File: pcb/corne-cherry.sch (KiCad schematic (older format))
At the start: 145 parts, among them J1 MJ-4PP-9, J2 OLED, J3 MJ-4PP-9, J4 OLED, J5 Conn_01x01_Male, J6 Conn_01x01_Male, P1 Conn_01x03, P3 Conn_01x03, SW1 SW_PUSH, SW10 SW_PUSH, SW11 SW_PUSH, SW12 SW_PUSH, SW13 SW_PUSH, SW14 SW_PUSH, SW15 SW_PUSH, SW16 SW_PUSH, SW17 SW_PUSH, SW18 SW_PUSH, SW19 SW_PUSH, SW2 SW_PUSH, SW20 SW_PUSH, SW21 SW_PUSH, SW22 SW_PUSH, SW23 SW_PUSH, SW24 SW_PUSH, SW25 SW_PUSH, SW26 SW_PUSH, SW27 SW_PUSH, SW28 SW_PUSH, SW29 SW_PUSH, SW3 SW_PUSH, SW30 SW_PUSH, SW31 SW_PUSH, SW32 SW_PUSH, SW33 SW_PUSH, SW34 SW_PUSH, SW35 SW_PUSH, SW36 SW_PUSH, SW37 SW_PUSH, SW38 SW_PUSH, SW39 SW_PUSH, SW4 SW_PUSH, SW40 SW_PUSH, SW41 SW_PUSH, SW42 SW_PUSH, SW43 Rotary_Encoder_Switch, SW5 SW_PUSH, SW6 SW_PUSH, SW7 SW_PUSH, SW8 SW_PUSH, SW9 SW_PUSH, U1 ProMicro, U2 ProMicro

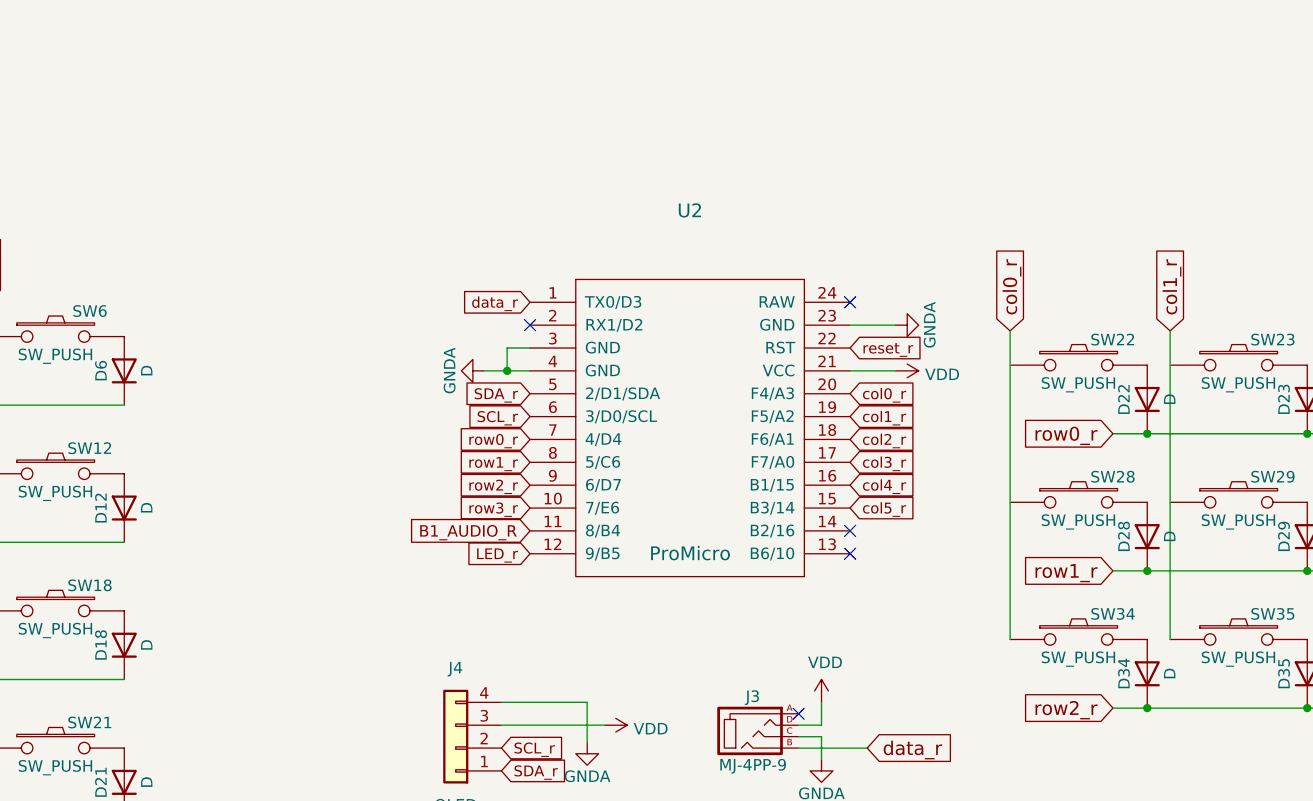
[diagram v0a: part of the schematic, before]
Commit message: Finish PCB
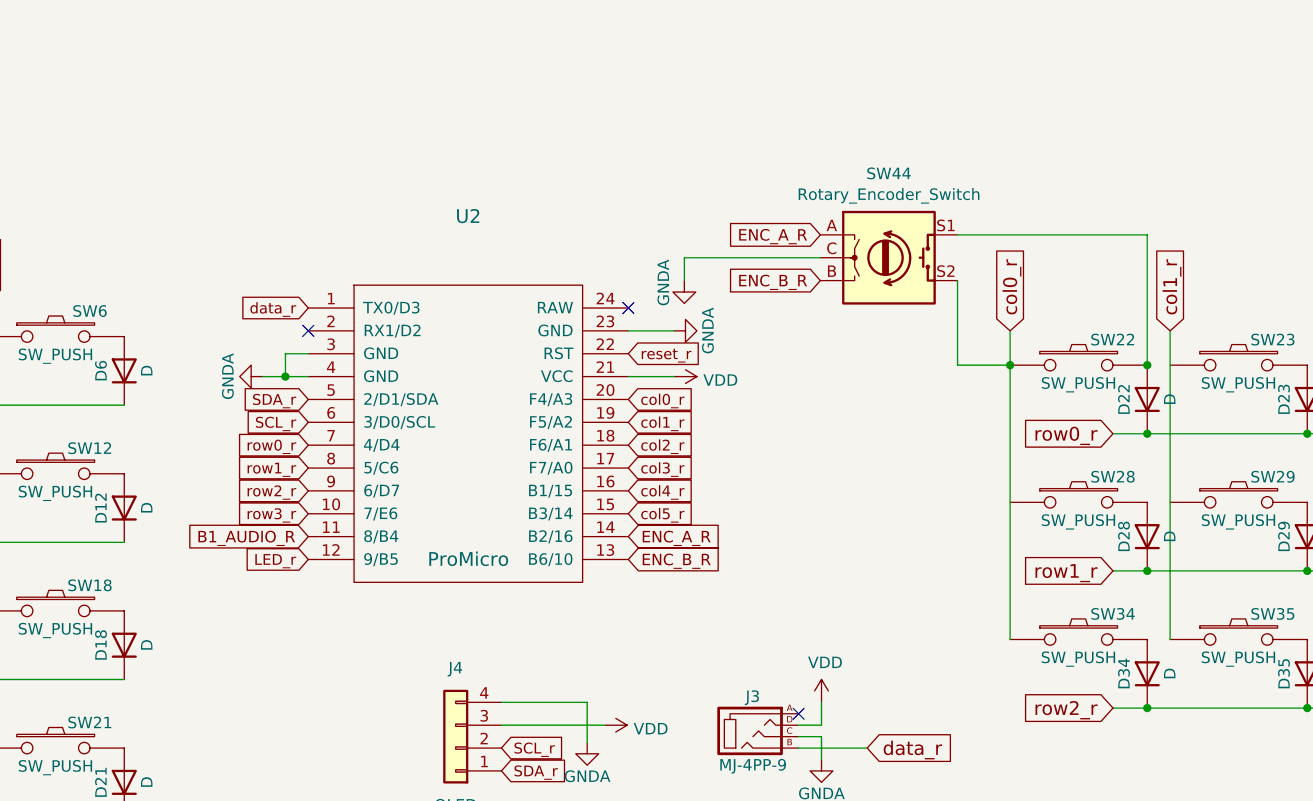
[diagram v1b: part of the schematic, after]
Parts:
- added SW44: Rotary_Encoder_Switch, Keebio-Parts:RotaryEncoder_EC11-no-legs, symbol Device:Rotary_Encoder_Switch
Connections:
- net GNDA: now also SW44.C
- net col0_r: now also SW22.1, SW44.S2
- net ENC_B_R: now reaches U2.13 (B6/10)
- net ENC_B_R: now also SW44.B
- net ENC_A_R: now reaches U2.14 (B2/16)
- net ENC_A_R: now also SW44.A
- net at D22.2 (A), SW22.2: now also SW44.S1
- no-connect marks 13 -> 11
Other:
- moved on the sheet: U2
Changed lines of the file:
@@
 L power:GNDA #PWR017
 U 1 1 5C25F963
-P 11075 1225
-F 0 "#PWR017" H 11075 975 50  0001 C CNN
-F 1 "GNDA" H 11075 1075 50  0000 C CNN
-F 2 "" H 11075 1225 50  0001 C CNN
-F 3 "" H 11075 1225 50  0001 C CNN
-	1    11075 1225
+P 10105 1250
+F 0 "#PWR017" H 10105 1000 50  0001 C CNN
+F 1 "GNDA" H 10105 1100 50  0000 C CNN
+F 2 "" H 10105 1250 50  0001 C CNN
+F 3 "" H 10105 1250 50  0001 C CNN
+	1    10105 1250
 	0    -1   -1   0
 $EndComp
@@
 L power:GNDA #PWR018
 U 1 1 5C25F969
-P 9275 1425
-F 0 "#PWR018" H 9275 1175 50  0001 C CNN
-F 1 "GNDA" H 9275 1275 50  0000 C CNN
-F 2 "" H 9275 1425 50  0001 C CNN
-F 3 "" H 9275 1425 50  0001 C CNN
-	1    9275 1425
+P 8305 1450
+F 0 "#PWR018" H 8305 1200 50  0001 C CNN
+F 1 "GNDA" H 8305 1300 50  0000 C CNN
+F 2 "" H 8305 1450 50  0001 C CNN
+F 3 "" H 8305 1450 50  0001 C CNN
+	1    8305 1450
 	0    1    1    0
 $EndComp
-Text GLabel 10875 1625 2    47   Input ~ 0
+Text GLabel 9905 1650 2    47   Input ~ 0
 col1_r
-Text GLabel 10875 1725 2    47   Input ~ 0
+Text GLabel 9905 1750 2    47   Input ~ 0
 col2_r
-Text GLabel 10875 1825 2    47   Input ~ 0
+Text GLabel 9905 1850 2    47   Input ~ 0
 col3_r
-Text GLabel 10875 1925 2    47   Input ~ 0
+Text GLabel 9905 1950 2    47   Input ~ 0
 col4_r
-Text GLabel 10875 2025 2    47   Input ~ 0
+Text GLabel 9905 2050 2    47   Input ~ 0
 col5_r
-Text GLabel 9475 2025 0    47   Input ~ 0
+Text GLabel 8505 2050 0    47   Input ~ 0
 row3_r
-Text GLabel 9475 1925 0    47   Input ~ 0
+Text GLabel 8505 1950 0    47   Input ~ 0
 row2_r
-Text GLabel 9475 1825 0    47   Input ~ 0
+Text GLabel 8505 1850 0    47   Input ~ 0
 row1_r
-Text GLabel 9475 1725 0    47   Input ~ 0
+Text GLabel 8505 1750 0    47   Input ~ 0
 row0_r
 $Comp
@@
 	1    0    0    -1
 $EndComp
-Text GLabel 9475 2225 0    47   Input ~ 0
+Text GLabel 8505 2250 0    47   Input ~ 0
 LED_r
-Text GLabel 9475 1125 0    47   Input ~ 0
+Text GLabel 8505 1150 0    47   Input ~ 0
 data_r
 $Comp
@@
 Text GLabel 10950 3075 2    60   Input ~ 0
 data_r
-Text GLabel 10875 1325 2    47   Input ~ 0
+Text GLabel 9905 1350 2    47   Input ~ 0
 reset_r
 Text GLabel 9375 3900 0    60   Input ~ 0
 reset_r
-NoConn ~ 9475 1225
-Text GLabel 10875 1525 2    47   Input ~ 0
+NoConn ~ 8505 1250
+Text GLabel 9905 1550 2    47   Input ~ 0
 col0_r
-NoConn ~ 10875 2125
-Text GLabel 9475 1525 0    47   Input ~ 0
+Text GLabel 8505 1550 0    47   Input ~ 0
 SDA_r
-Text GLabel 9475 1625 0    47   Input ~ 0
+Text GLabel 8505 1650 0    47   Input ~ 0
 SCL_r
 $Comp
@@
 Text GLabel 9350 3175 2    47   Input ~ 0
 SDA_r
-NoConn ~ 10875 1125
+NoConn ~ 9905 1150
 $Comp
 L kbd:MJ-4PP-9 J3
@@
 	12025 1700 12175 1700
 Wire Wire Line
-	9375 1325 9375 1425
-Connection ~ 9375 1425
-Wire Wire Line
-	9475 1325 9375 1325
-Wire Wire Line
-	9275 1425 9375 1425
+	8405 1350 8405 1450
+Connection ~ 8405 1450
+Wire Wire Line
+	8505 1350 8405 1350
+Wire Wire Line
+	8305 1450 8405 1450
 Connection ~ 12175 2900
 Connection ~ 12875 2900
@@
 Connection ~ 14975 1700
 Wire Wire Line
-	10875 1225 11075 1225
-Wire Wire Line
-	10875 1425 11075 1425
+	9905 1250 10105 1250
+Wire Wire Line
+	9905 1450 10105 1450
 Wire Wire Line
 	10650 3075 10950 3075
@@
 	14975 3500 15675 3500
 Wire Wire Line
-	9375 1425 9475 1425
+	8405 1450 8505 1450
 Wire Wire Line
 	12175 2900 12875 2900
@@
 L power:VDD #PWR019
 U 1 1 5C714C7F
-P 11075 1425
-F 0 "#PWR019" H 11075 1275 50  0001 C CNN
-F 1 "VDD" V 11092 1553 50  0000 L CNN
-F 2 "" H 11075 1425 50  0001 C CNN
-F 3 "" H 11075 1425 50  0001 C CNN
-	1    11075 1425
+P 10105 1450
+F 0 "#PWR019" H 10105 1300 50  0001 C CNN
+F 1 "VDD" V 10122 1578 50  0000 L CNN
+F 2 "" H 10105 1450 50  0001 C CNN
+F 3 "" H 10105 1450 50  0001 C CNN
+	1    10105 1450
 	0    1    1    0
 $EndComp
@@
 	5000 1125 5000 2475
 Wire Wire Line
-	11575 1250 11575 2600
+	11575 1250 11575 1400
 Wire Wire Line
 	12275 1250 12275 2600
@@
 L kbd:ProMicro U2
 U 1 1 5C25F857
-P 10175 1675
-F 0 "U2" H 10175 2625 60  0000 C CNN
-F 1 "ProMicro" H 10175 1125 60  0000 C CNN
-F 2 "kbd:ProMicro_v3" H 10275 625 60  0001 C CNN
-F 3 "" H 10275 625 60  0000 C CNN
-	1    10175 1675
-	1    0    0    -1
-$EndComp
-NoConn ~ 10875 2225
+P 9205 1700
+F 0 "U2" H 9205 2650 60  0000 C CNN
+F 1 "ProMicro" H 9205 1150 60  0000 C CNN
+F 2 "kbd:ProMicro_v3" H 9305 650 60  0001 C CNN
+F 3 "" H 9305 650 60  0000 C CNN
+	1    9205 1700
+	1    0    0    -1
+$EndComp
 NoConn ~ 5718 9687
 NoConn ~ 5470 8376
@@
 Wire Wire Line
 	7467 8158 7467 8302
-Text GLabel 9475 2125 0    50   Input ~ 0
+Text GLabel 8505 2150 0    50   Input ~ 0
 B1_AUDIO_R
 Text GLabel 1712 7647 2    50   Input ~ 0
@@
 	2420 785  2420 885
 $Comp
-L power:GND #PWR?
+L power:GND #PWR0119
 U 1 1 60823858
 P 2420 885
-F 0 "#PWR?" H 2420 635 50  0001 C CNN
+F 0 "#PWR0119" H 2420 635 50  0001 C CNN
 F 1 "GND" H 2425 712 50  0000 C CNN
 F 2 "" H 2420 885 50  0001 C CNN
@@
 	4200 685  4200 1275
 Connection ~ 4200 1275
+Text GLabel 9905 2150 2    50   Input ~ 0
+ENC_A_R
+Text GLabel 9905 2250 2    50   Input ~ 0
+ENC_B_R
+$Comp
+L Device:Rotary_Encoder_Switch SW44
+U 1 1 60786552
+P 11045 930
+F 0 "SW44" H 11045 1297 50  0000 C CNN
+F 1 "Rotary_Encoder_Switch" H 11045 1206 50  0000 C CNN
+F 2 "Keebio-Parts:RotaryEncoder_EC11-no-legs" H 10895 1090 50  0001 C CNN
+F 3 "~" H 11045 1190 50  0001 C CNN
+	1    11045 930
+	1    0    0    -1
+$EndComp
+Text GLabel 10745 1030 0    50   Input ~ 0
+ENC_B_R
+Text GLabel 10745 830  0    50   Input ~ 0
+ENC_A_R
+Wire Wire Line
+	10745 930  10150 930
+Wire Wire Line
+	10150 930  10150 1030
+$Comp
+L power:GNDA #PWR0120
+U 1 1 607DCD43
+P 10150 1030
+F 0 "#PWR0120" H 10150 780 50  0001 C CNN
+F 1 "GNDA" V 10060 1020 50  0000 C CNN
+F 2 "" H 10150 1030 50  0001 C CNN
+F 3 "" H 10150 1030 50  0001 C CNN
+	1    10150 1030
+	1    0    0    -1
+$EndComp
+Wire Wire Line
+	11345 830  12175 830
+Wire Wire Line
+	12175 830  12175 1400
+Connection ~ 12175 1400
+Wire Wire Line
+	11345 1030 11345 1400
+Wire Wire Line
+	11345 1400 11575 1400
+Connection ~ 11575 1400
+Wire Wire Line
+	11575 1400 11575 2600
 $EndSCHEMATC
